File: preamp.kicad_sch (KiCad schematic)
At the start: 18 parts, among them Q1 2N3904, Q2 2N3904

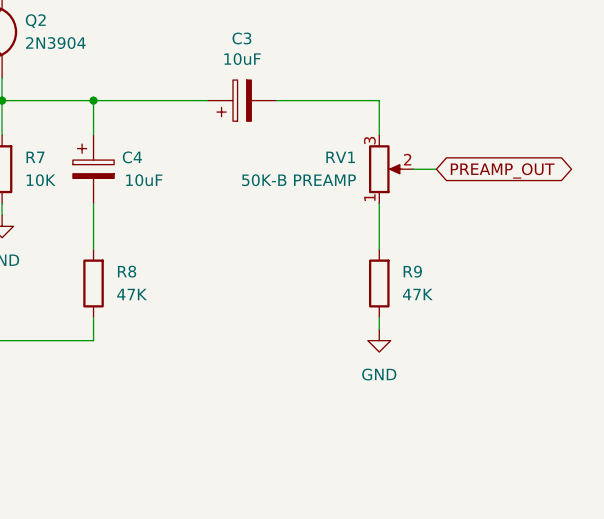
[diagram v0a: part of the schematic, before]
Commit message: Archivos de Fabricación listos.
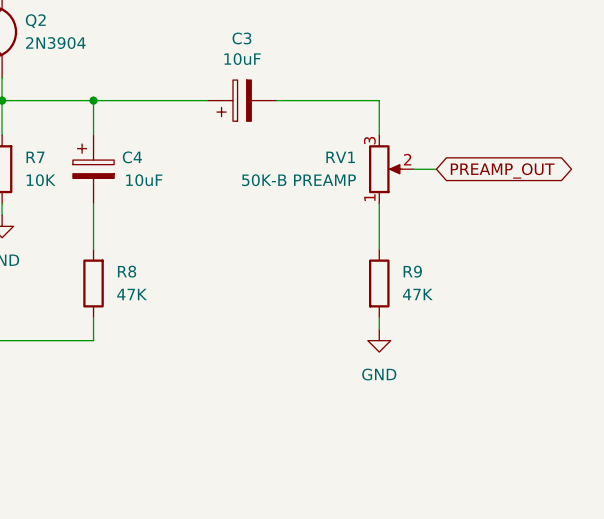
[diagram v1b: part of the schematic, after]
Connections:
- net GND: now also R9.2; no longer R9.1
- net at RV1.1: now also R9.1; no longer R9.2
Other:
- moved on the sheet: R9
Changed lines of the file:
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@@
 	(symbol
 		(lib_id "Device:R")
-		(at 194.31 116.84 180)
+		(at 194.31 116.84 0)
 		(unit 1)
 		(exclude_from_sim no)
@@
 		(fields_autoplaced yes)
 		(property "Reference" "R9"
-			(at 196.85 115.57 0)
+			(at 196.85 115.5699 0)
 			(effects
 				(font
 					(size 1.27 1.27)
 				)
-				(justify right)
+				(justify left)
 			)
 		)
 		(property "Value" "47K"
-			(at 196.85 118.11 0)
+			(at 196.85 118.1099 0)
 			(effects
 				(font
 					(size 1.27 1.27)
 				)
-				(justify right)
+				(justify left)
 			)
 		)
 		(property "Footprint" "Resistor_THT:R_Axial_DIN0207_L6.3mm_D2.5mm_P7.62mm_Horizontal"
-			(at 196.088 116.84 90)
+			(at 192.532 116.84 90)
 			(effects
 				(font
